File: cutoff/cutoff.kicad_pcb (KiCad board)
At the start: 2 copper layers, 137 x 76 mm, 28 parts, among them J1 Conn_01x01, J10 Conn_01x01, J11 Conn_01x01, J12 Conn_01x01, J13 Conn_01x01, J14 Conn_01x01, J15 Conn_01x01, J2 Conn_01x01, J3 Conn_01x01, J4 Conn_01x01, J5 Conn_01x01, J6 Conn_01x01, J7 Conn_01x01, J8 Conn_01x01, J9 Conn_01x01, U1 TPS3700DDCR, U2 BTS50010-1TAD

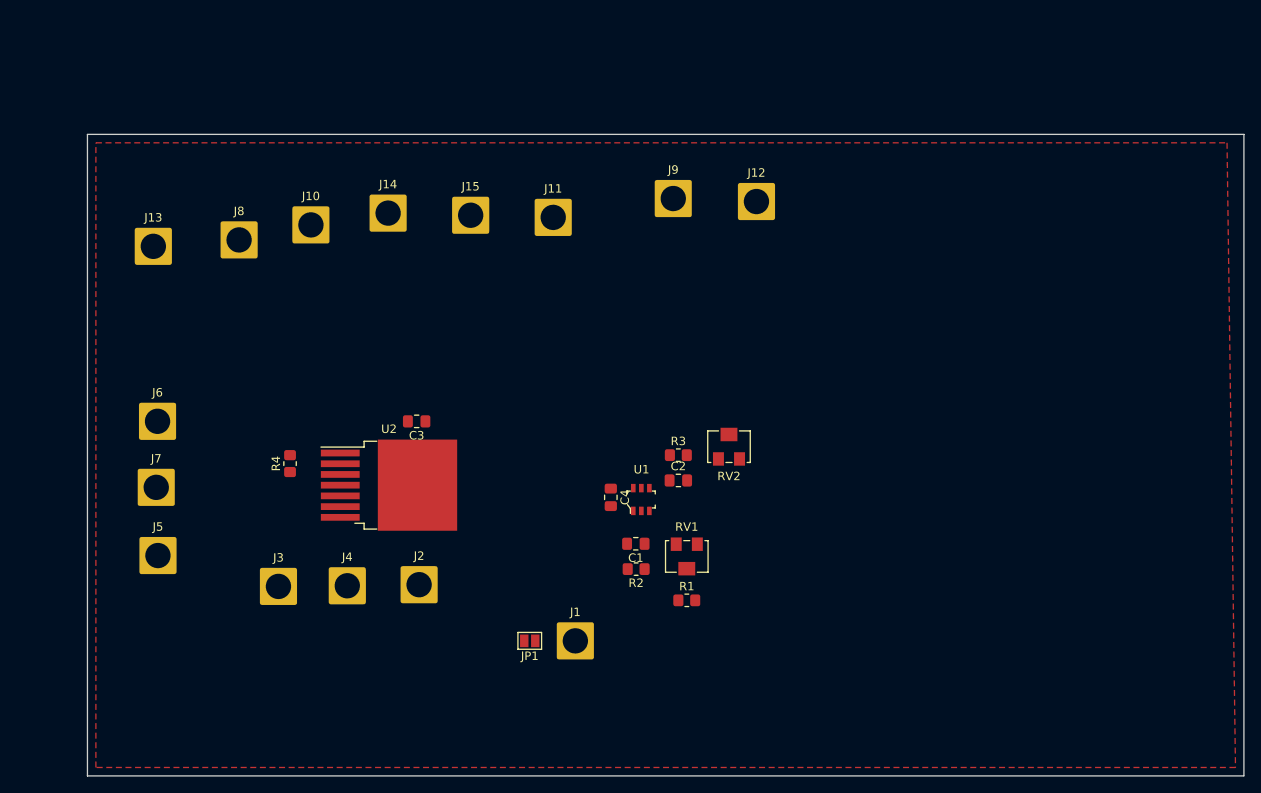
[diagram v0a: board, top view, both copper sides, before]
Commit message: wip
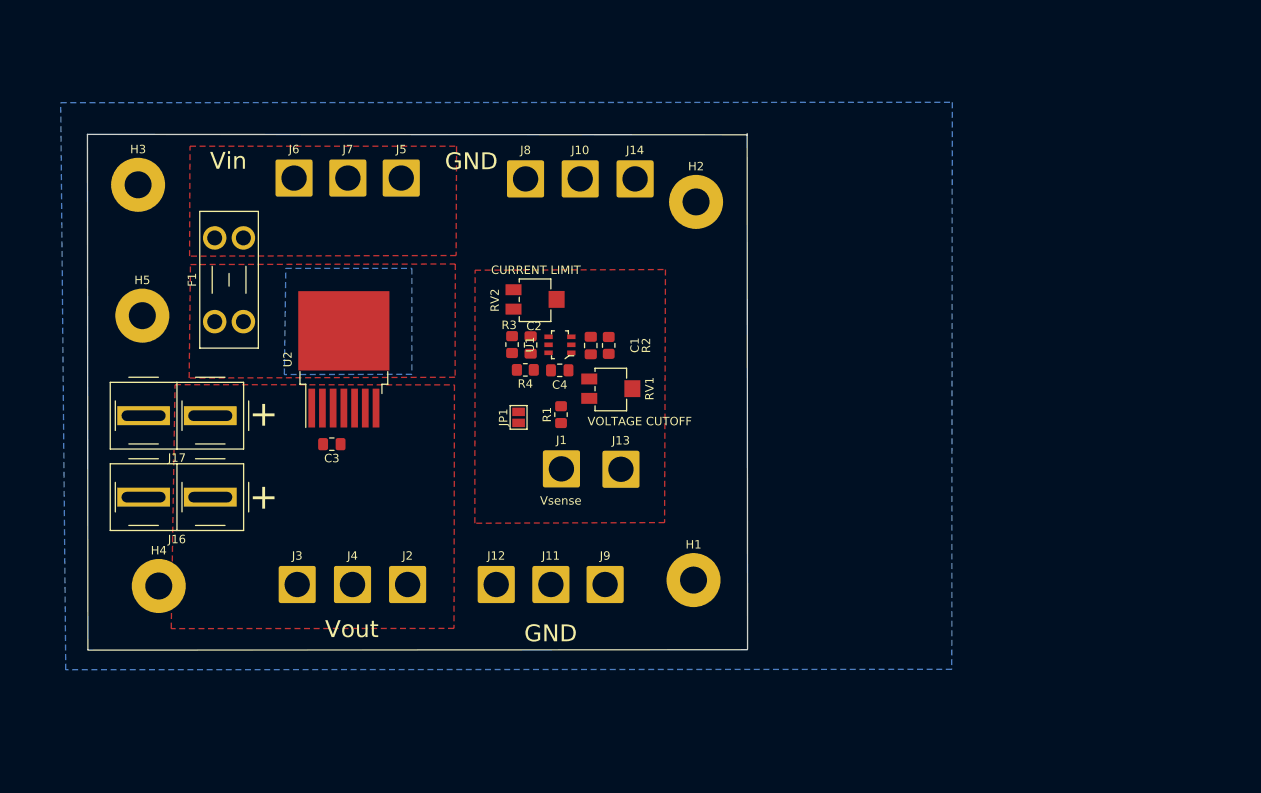
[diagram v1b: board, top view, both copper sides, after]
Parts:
- removed J15: Conn_01x01, Connector_Wire:SolderWire-2.5sqmm_1x01_D2.4mm_OD4.4mm
- added F1: Fuse, Fuse:Fuseholder_Blade_Mini_Keystone_3568, F.Cu at (64.1, 51.2)
- added H1: MountingHole_Pad, MountingHole:MountingHole_3.2mm_M3_Pad, F.Cu at (120.8, 81.8)
- added H2: MountingHole_Pad, MountingHole:MountingHole_3.2mm_M3_Pad, F.Cu at (121.1, 37.0)
- added H3: MountingHole_Pad, MountingHole:MountingHole_3.2mm_M3_Pad, F.Cu at (55.0, 35.0)
- added H4: MountingHole_Pad, MountingHole:MountingHole_3.2mm_M3_Pad, F.Cu at (57.5, 82.5)
- added H5: MountingHole_Pad, MountingHole:MountingHole_3.2mm_M3_Pad, F.Cu at (55.5, 50.5)
- added J16: Conn_01x02, connectors_anderson:45A-VERT-PAIR, F.Cu at (59.6, 72.0)
- added J17: Conn_01x02, connectors_anderson:45A-VERT-PAIR, F.Cu at (59.6, 62.3)
- RV1, RV2: footprint Potentiometer_SMD:Potentiometer_Bourns_3224W_Vertical -> Potentiometer_SMD:Potentiometer_Bourns_3224X_Vertical
- moved J13 61.4 mm to (112.2, 68.7)
- moved J12 54.9 mm to (97.4, 82.3)
- moved J5 53.2 mm to (86.2, 34.2)
- moved J9 46.4 mm to (110.3, 82.3)
- moved J11 43.5 mm to (103.9, 82.3)
- moved J7 43.1 mm to (79.8, 34.2)
- moved J8 34.7 mm to (100.9, 34.3)
- moved J6 33.0 mm to (73.5, 34.2)
- moved J10 32.4 mm to (107.4, 34.3)
- moved R4 30.0 mm to (100.9, 56.9), turned to 180 degrees
- moved J14 29.5 mm to (113.9, 34.3)
- moved RV2 28.9 mm to (102.0, 48.5), turned to 90 degrees
- moved R2 26.7 mm to (110.8, 54.0), turned to -90 degrees
- moved R1 26.6 mm to (105.1, 62.2), turned to 90 degrees
- moved JP1 26.5 mm to (100.1, 62.5), turned to 90 degrees
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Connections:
- net Net-(C2-Pad1) renamed /Vis
- net Net-(J1-Pad1) renamed /Vsense
- net Net-(J2-Pad1) renamed /OUT
- net Net-(RV1-Pad2) renamed /Vcut
- J5 pad 1: VDD -> /VIN
- J6 pad 1: VDD -> /VIN
- J7 pad 1: VDD -> /VIN
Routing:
- added copper zone on F.Cu, net /VIN
- added copper zone on B.Cu, net GND
- added copper zone on F.Cu, net Net-(J16-Pad1)
- added copper zone on B.Cu, net VDD
- added copper zone on F.Cu, net VDD
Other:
- board size 137 x 76 mm -> 78.2 x 61.2 mm
- board text added: "+"
- board text added: "CURRENT LIMIT"
- board text added: "GND"
- board text added: "VOLTAGE CUTOFF"
- board text added: "Vin"
- board text added: "Vout"
- board text added: "Vsense"

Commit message: wip
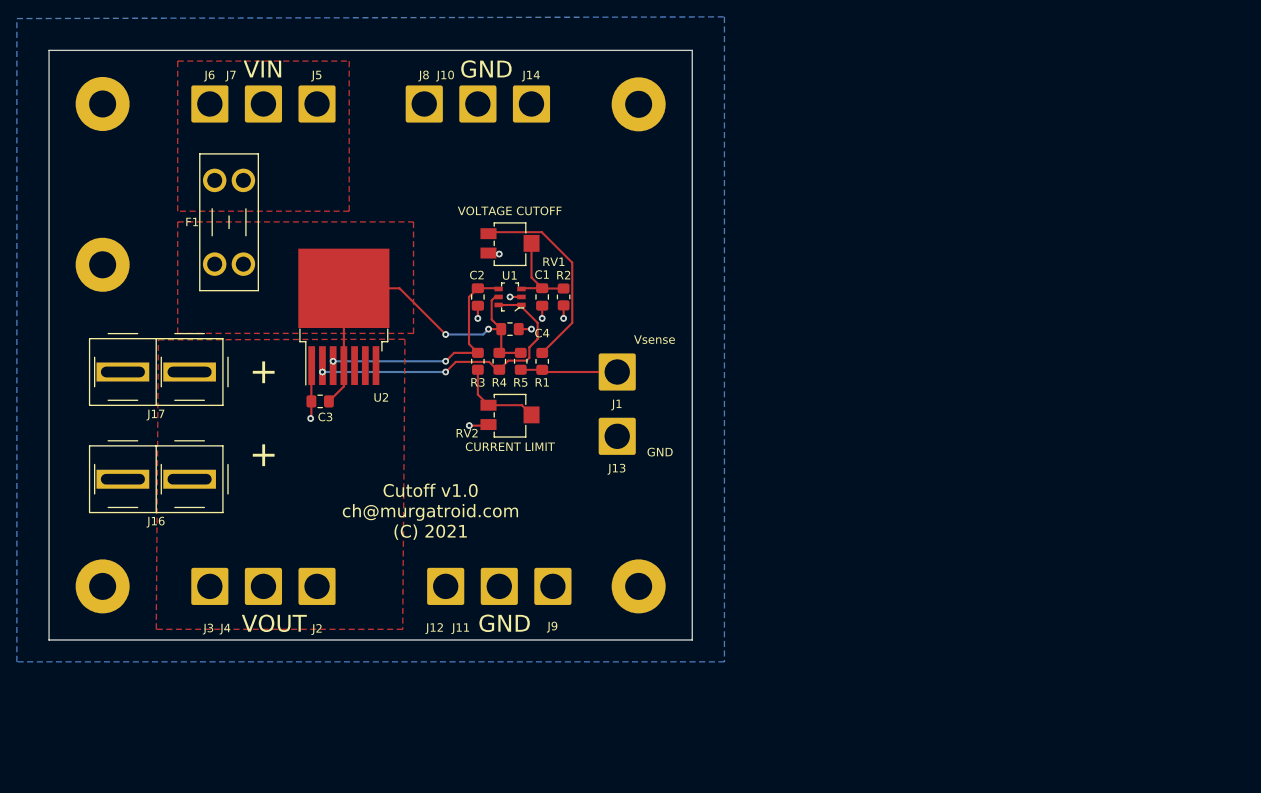
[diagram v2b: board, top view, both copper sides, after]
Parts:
- removed JP1: SolderJumper_2_Open, Jumper:SolderJumper-2_P1.3mm_Open_Pad1.0x1.5mm
- added R5: *0, Resistor_SMD:R_0805_2012Metric_Pad1.20x1.40mm_HandSolder, F.Cu at (100.3, 55.9)
- moved RV1 21.0 mm to (99.1, 41.9)
- moved J14 15.1 mm to (101.6, 25.4)
- moved J10 15.0 mm to (95.2, 25.4)
- moved J8 14.9 mm to (88.9, 25.4)
- moved RV2 14.0 mm to (99.1, 62.2)
- moved H2 13.4 mm to (114.3, 25.4)
- moved J7 13.3 mm to (69.8, 25.4)
- moved J5 13.3 mm to (76.2, 25.4)
- moved J6 13.3 mm to (63.5, 25.4)
- moved J1 13.2 mm to (111.8, 57.1)
- moved J2 10.7 mm to (76.2, 82.5)
- moved J4 10.6 mm to (69.8, 82.5)
- moved H3 10.5 mm to (50.8, 25.4)
- moved J3 10.4 mm to (63.5, 82.5)
- moved C2 8.45 mm to (95.2, 48.3)
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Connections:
- net /Vcut renamed /Voff
- net /Vis renamed /IS
- net Net-(R4-Pad2) renamed /EN
- J16 pad 1: Net-(J16-Pad1) -> /OUT
- J17 pad 1: Net-(J16-Pad1) -> /OUT
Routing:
- net VDD: track 0.00 -> 45.3 mm, vias 0 -> 2
- net /EN: track 0.00 -> 35.9 mm, vias 0 -> 2
- net /IS: track 0.00 -> 28.5 mm, vias 0 -> 2
- net Net-(R1-Pad2): track 0.00 -> 23.4 mm
- net GND: track 0.00 -> 17.0 mm, vias 0 -> 8
- net /Vsense: track 0.00 -> 11.2 mm
- net /Voff: track 0.00 -> 10.7 mm
- net Net-(R3-Pad2): track 0.00 -> 10.3 mm
- added copper zone on F.Cu, net /OUT
- removed copper zone on F.Cu, net GND
- removed copper zone on F.Cu, net Net-(J16-Pad1)
- removed copper zone on B.Cu, net VDD
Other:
- board size 78.2 x 61.2 mm -> 76.2 x 69.9 mm
- board text added: "Cutoff v1.0 ch@murgatroid.com (C) 2021"
- board text added: "VIN"
- board text added: "VOUT"
- board text removed: "Vin"
- board text removed: "Vout"
